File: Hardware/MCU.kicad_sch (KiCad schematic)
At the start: 13 parts, among them J2 Debug, U6 CW32F030K8

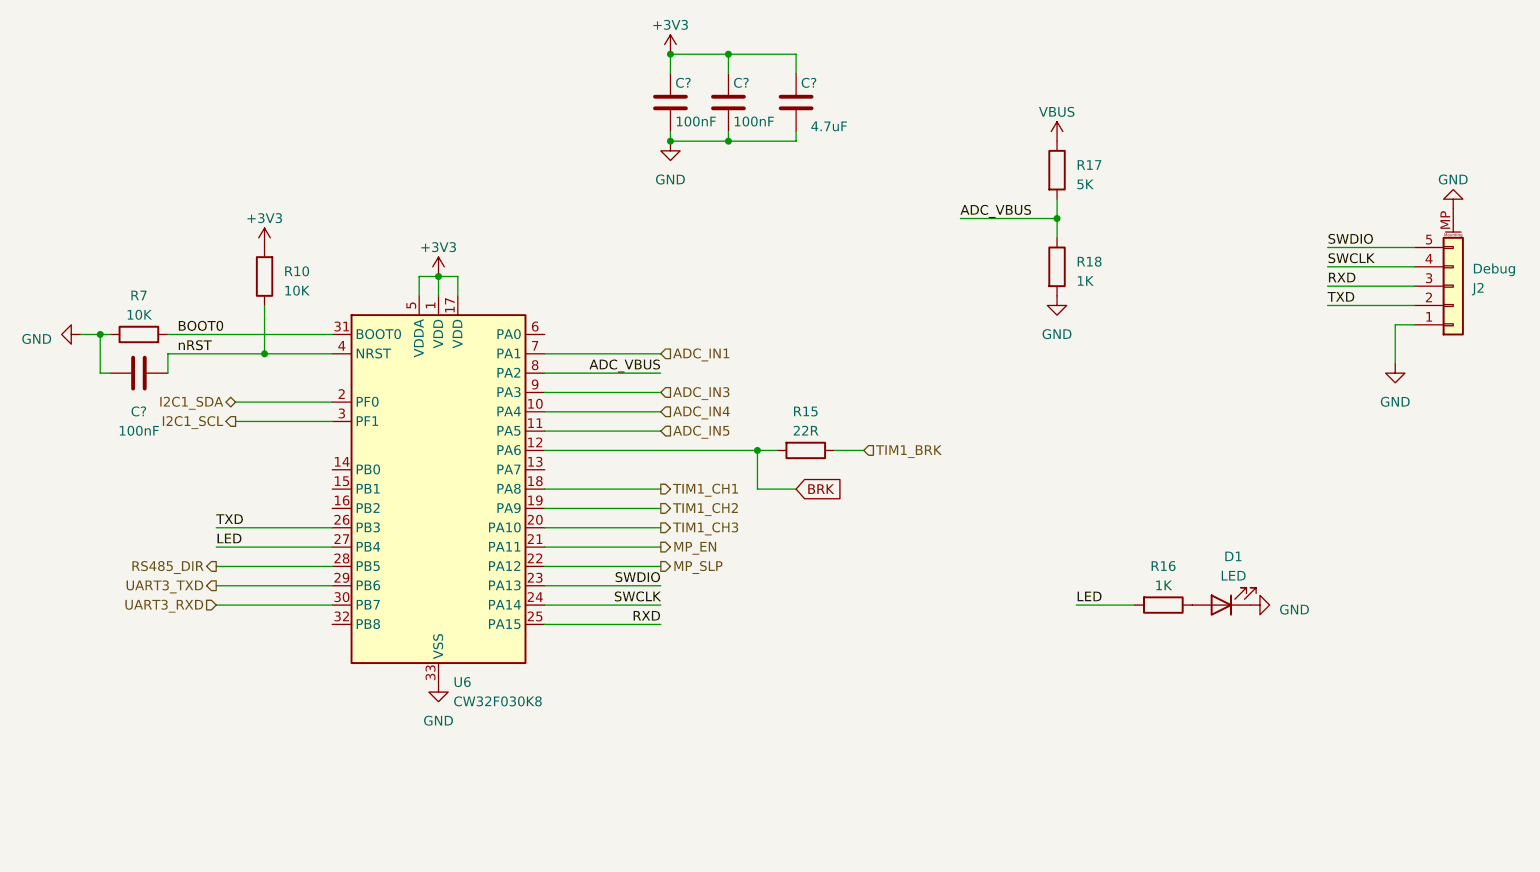
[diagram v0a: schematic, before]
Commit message: 第一版硬件做好啦！(●'◡'●)
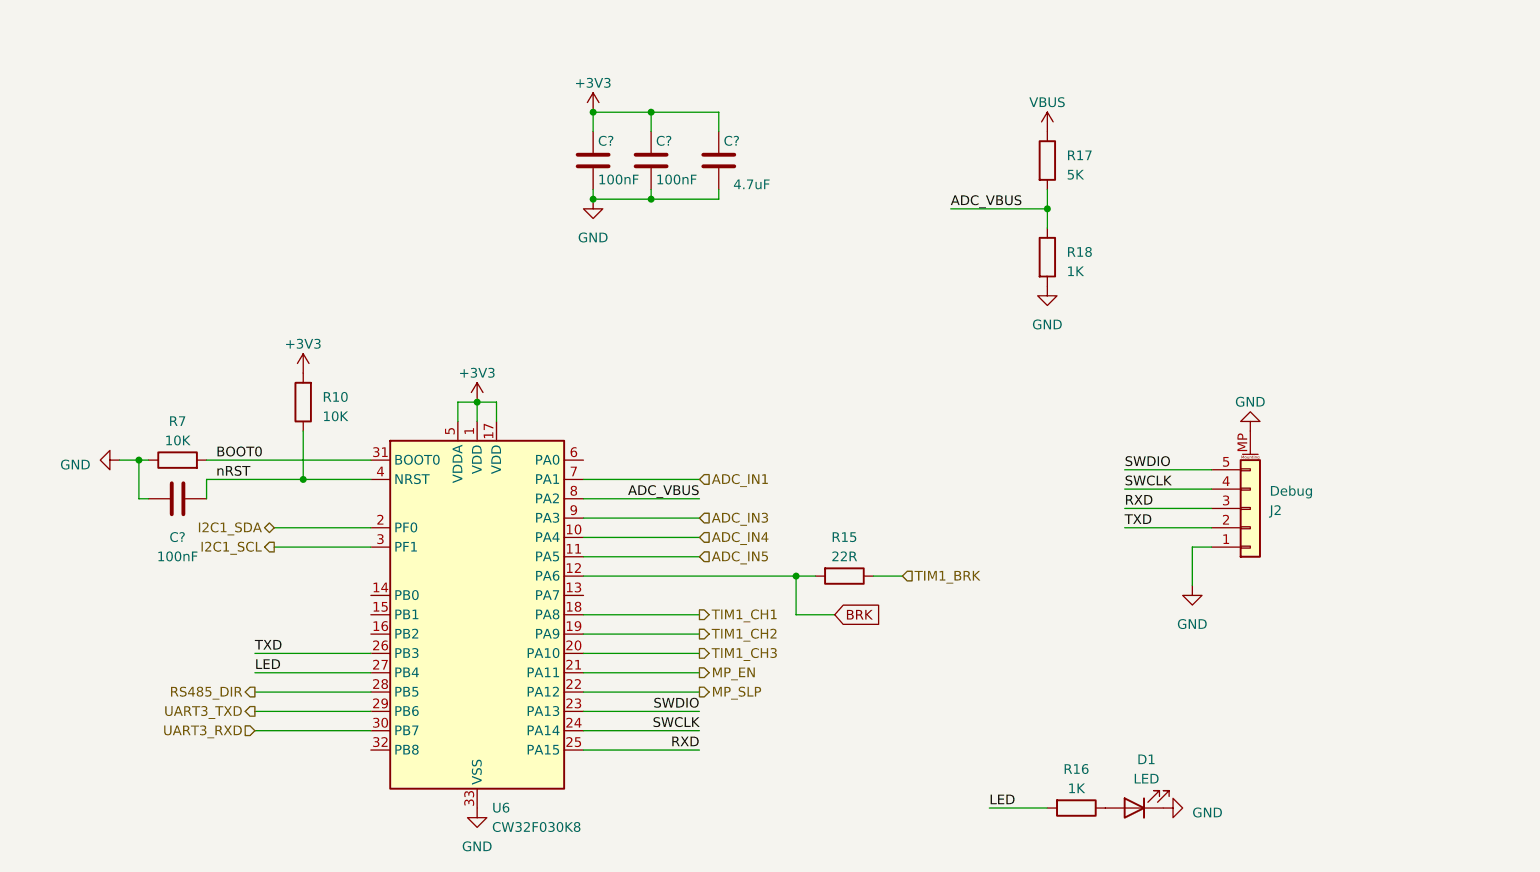
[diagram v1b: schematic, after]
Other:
- company: (none) -> Akako Industry
- title: (none) -> cwFOC/MCU
- moved on the sheet: C?, D1, J2, R10, R15, R16, R17, R18, R7, U6

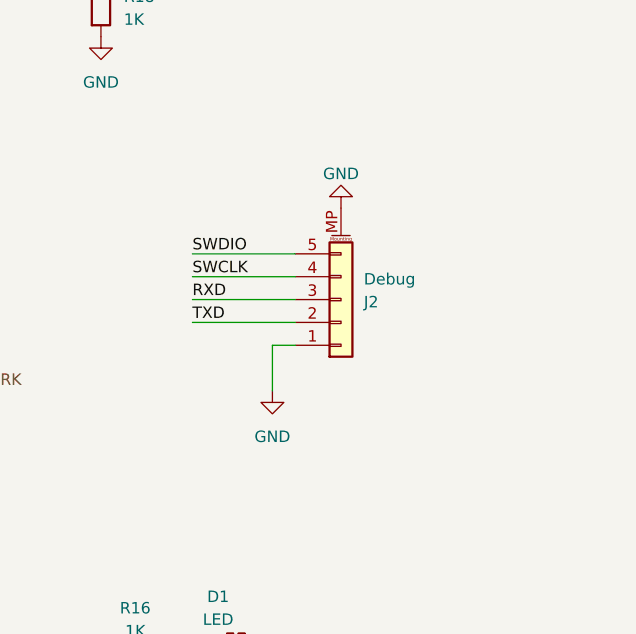
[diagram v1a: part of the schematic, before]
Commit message: 调整第二版原理图
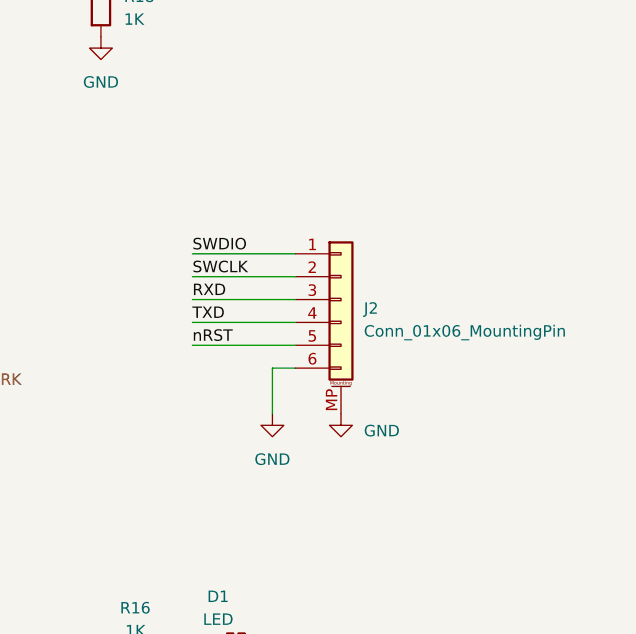
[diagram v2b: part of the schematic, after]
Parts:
- removed J2: Debug, Connector_JST:JST_SH_BM05B-SRSS-TB_1x05-1MP_P1.00mm_Vertical, symbol Connector_Generic_MountingPin:Conn_01x05_MountingPin
- added J2: Conn_01x06_MountingPin, Connector_JST:JST_GH_SM06B-GHS-TB_1x06-1MP_P1.25mm_Horizontal, symbol Connector_Generic_MountingPin:Conn_01x06_MountingPin
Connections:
- net GND: now also J2.6 (Pin_6), J2.MP (MountPin)
- net RXD: now also J2.3 (Pin_3)
- net SWCLK: now also J2.2 (Pin_2)
- net SWDIO: now also J2.1 (Pin_1)
- net TXD: now also J2.4 (Pin_4)
- net nRST: now also J2.5 (Pin_5)
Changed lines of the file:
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@@
+    (stroke (width 0) (type default))
+  )
+  (wire (pts (xy 200.66 110.49) (xy 212.09 110.49))
     (stroke (width 0) (type default))
   )
@@
     (stroke (width 0) (type default))
   )
-  (wire (pts (xy 212.09 110.49) (xy 209.55 110.49))
+  (wire (pts (xy 212.09 113.03) (xy 209.55 113.03))
     (stroke (width 0) (type default))
   )
@@
     (stroke (width 0) (type default))
   )
-  (wire (pts (xy 209.55 110.49) (xy 209.55 115.57))
+  (wire (pts (xy 209.55 113.03) (xy 209.55 118.11))
     (stroke (width 0) (type default))
   )
@@
   )
   (label "BOOT0" (at 81.28 99.06 0) (fields_autoplaced)
+    (effects (font (size 1.27 1.27)) (justify left bottom))
+  )
+  (label "nRST" (at 200.66 110.49 0) (fields_autoplaced)
     (effects (font (size 1.27 1.27)) (justify left bottom))
   )
@@
     )
   )
+  (symbol (lib_id "Connector_Generic_MountingPin:Conn_01x06_MountingPin") (at 217.17 105.41 0) (unit 1)
+    (in_bom yes) (on_board yes) (dnp no) (fields_autoplaced)
+    (property "Reference" "J2" (at 219.71 106.4006 0)
+      (effects (font (size 1.27 1.27)) (justify left))
+    )
+    (property "Value" "Conn_01x06_MountingPin" (at 219.71 108.9406 0)
+      (effects (font (size 1.27 1.27)) (justify left))
+    )
+    (property "Footprint" "Connector_JST:JST_GH_SM06B-GHS-TB_1x06-1MP_P1.25mm_Horizontal" (at 217.17 105.41 0)
+      (effects (font (size 1.27 1.27)) hide)
+    )
+    (property "Datasheet" "~" (at 217.17 105.41 0)
+      (effects (font (size 1.27 1.27)) hide)
+    )
+    (pin "1")
+    (pin "2")
+    (pin "3")
+    (pin "4")
+    (pin "5")
+    (pin "6")
+    (pin "MP")
+    (instances
+      (project "cwFOC"
+        (path "/ff847474-9801-42c6-af12-b4b1b75aa0af/1a00d99a-20c9-415d-b828-323b0b58b185"
+          (reference "J2") (unit 1)
+        )
+      )
+    )
+  )
   (symbol (lib_id "power:VBUS") (at 190.5 55.88 0) (unit 1)
     (in_bom yes) (on_board yes) (dnp no) (fields_autoplaced)
@@
     )
   )
-  (symbol (lib_id "power:GND") (at 217.17 95.25 180) (unit 1)
-    (in_bom yes) (on_board yes) (dnp no) (fields_autoplaced)
-    (property "Reference" "#PWR041" (at 217.17 88.9 0)
-      (effects (font (size 1.27 1.27)) hide)
-    )
-    (property "Value" "GND" (at 217.17 91.44 0)
-      (effects (font (size 1.27 1.27)))
-    )
-    (property "Footprint" "" (at 217.17 95.25 0)
-      (effects (font (size 1.27 1.27)) hide)
-    )
-    (property "Datasheet" "" (at 217.17 95.25 0)
+  (symbol (lib_id "power:GND") (at 217.17 118.11 0) (unit 1)
+    (in_bom yes) (on_board yes) (dnp no) (fields_autoplaced)
+    (property "Reference" "#PWR041" (at 217.17 124.46 0)
+      (effects (font (size 1.27 1.27)) hide)
+    )
+    (property "Value" "GND" (at 219.71 120.015 0)
+      (effects (font (size 1.27 1.27)) (justify left))
+    )
+    (property "Footprint" "" (at 217.17 118.11 0)
+      (effects (font (size 1.27 1.27)) hide)
+    )
+    (property "Datasheet" "" (at 217.17 118.11 0)
       (effects (font (size 1.27 1.27)) hide)
     )
@@
     )
   )
-  (symbol (lib_id "power:GND") (at 209.55 115.57 0) (unit 1)
-    (in_bom yes) (on_board yes) (dnp no) (fields_autoplaced)
-    (property "Reference" "#PWR042" (at 209.55 121.92 0)
-      (effects (font (size 1.27 1.27)) hide)
-    )
-    (property "Value" "GND" (at 209.55 120.65 0)
-      (effects (font (size 1.27 1.27)))
-    )
-    (property "Footprint" "" (at 209.55 115.57 0)
-      (effects (font (size 1.27 1.27)) hide)
-    )
-    (property "Datasheet" "" (at 209.55 115.57 0)
+  (symbol (lib_id "power:GND") (at 209.55 118.11 0) (unit 1)
+    (in_bom yes) (on_board yes) (dnp no) (fields_autoplaced)
+    (property "Reference" "#PWR042" (at 209.55 124.46 0)
+      (effects (font (size 1.27 1.27)) hide)
+    )
+    (property "Value" "GND" (at 209.55 123.19 0)
+      (effects (font (size 1.27 1.27)))
+    )
+    (property "Footprint" "" (at 209.55 118.11 0)
+      (effects (font (size 1.27 1.27)) hide)
+    )
+    (property "Datasheet" "" (at 209.55 118.11 0)
       (effects (font (size 1.27 1.27)) hide)
     )
@@
         )
       )
-    )
-  )
-  (symbol (lib_id "Connector_Generic_MountingPin:Conn_01x05_MountingPin") (at 217.17 105.41 0) (mirror x) (unit 1)
-    (in_bom yes) (on_board yes) (dnp no)
-    (property "Reference" "J2" (at 219.71 105.6894 0)
-      (effects (font (size 1.27 1.27)) (justify left))
-    )
-    (property "Value" "Debug" (at 219.71 103.1494 0)
-      (effects (font (size 1.27 1.27)) (justify left))
-    )
-    (property "Footprint" "Connector_JST:JST_SH_BM05B-SRSS-TB_1x05-1MP_P1.00mm_Vertical" (at 217.17 105.41 0)
-      (effects (font (size 1.27 1.27)) hide)
-    )
-    (property "Datasheet" "~" (at 217.17 105.41 0)
-      (effects (font (size 1.27 1.27)) hide)
-    )
-    (pin "1")
-    (pin "2")
-    (pin "3")
-    (pin "4")
-    (pin "5")
-    (pin "MP")
-    (instances
-      (project "cwFOC"
-        (path "/ff847474-9801-42c6-af12-b4b1b75aa0af/1a00d99a-20c9-415d-b828-323b0b58b185"
-          (reference "J2") (unit 1)
-        )
-      )
